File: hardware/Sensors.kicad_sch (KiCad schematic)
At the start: 1 part, among them U107 LIS3DH

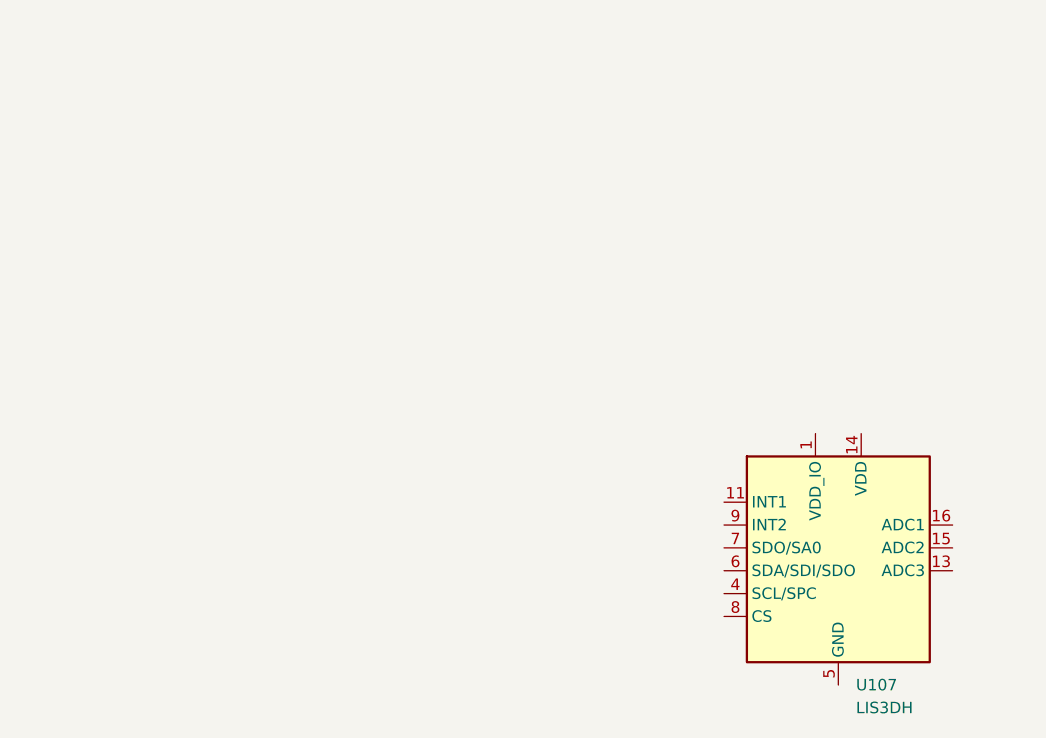
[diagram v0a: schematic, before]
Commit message: asdf
Signed-off-by: Connor Rigby <connorr@hey.com>
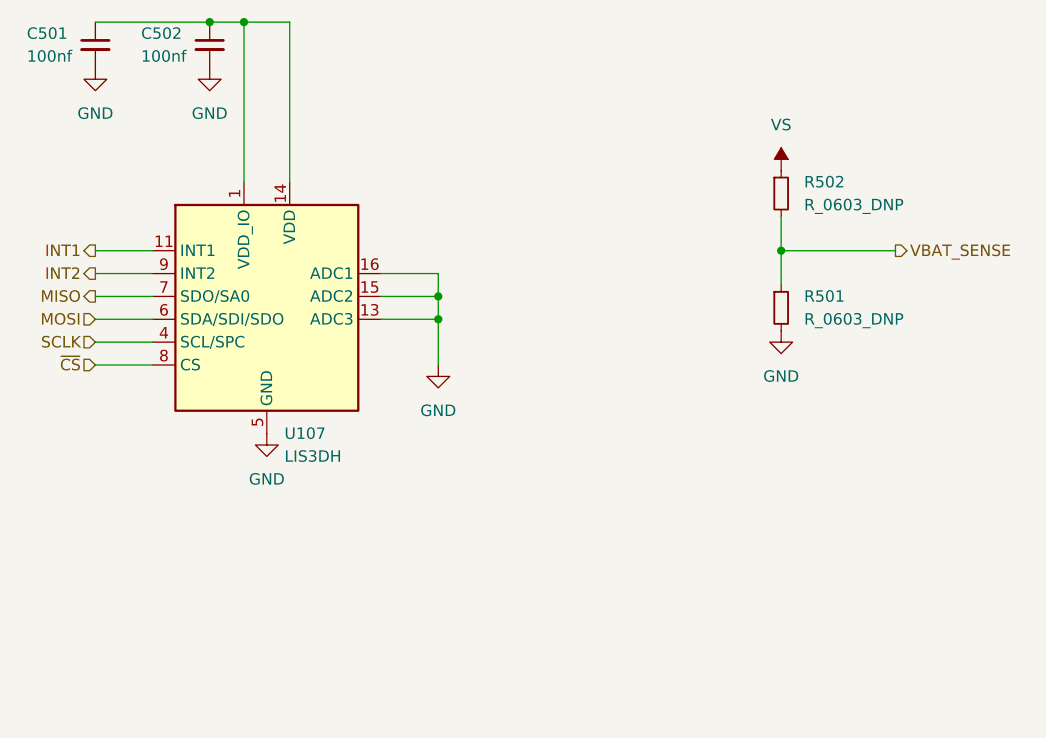
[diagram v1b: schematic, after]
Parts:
- added C501, C502: C_0402_100nf_X7R, Capacitor_SMD:C_0402_1005Metric, symbol LCSC_Capacitor:C_0402_100nf_X7R
- added R501, R502: R_0603_DNP, Resistor_SMD:R_0603_1608Metric, symbol LCSC_Resistor:R_0603_DNP
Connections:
- net at U107.1 (VDD_IO): now also U107.14 (VDD), C501.1, C502.1
- net GND: now reaches U107.10 (GND), U107.12 (GND), U107.5 (GND)
- net GND: now also U107.13 (ADC3), U107.15 (ADC2), U107.16 (ADC1), C501.2, C502.2, R501.2
- net INT1: now reaches U107.11 (INT1)
- net SCLK: now reaches U107.4 (SCL/SPC)
- net MOSI: now reaches U107.6 (SDA/SDI/SDO)
- net MISO: now reaches U107.7 (SDO/SA0)
- net ~{CS}: now reaches U107.8 (CS)
- net INT2: now reaches U107.9 (INT2)
- new net VBAT_SENSE: R501.1, R502.2
- new net VS: R502.1
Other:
- moved on the sheet: U107
